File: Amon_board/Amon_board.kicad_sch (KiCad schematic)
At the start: 40 parts, among them J1 USB2.0_C_Rev, J2 Conn_2x5 pin, SW1 SW_DPDT, SW2 SW_SPST, U1 USBLC6-2P6, U2 STM32F405RGT6-LQFP64, U3 W25Q128JVS, Y1 25MHz

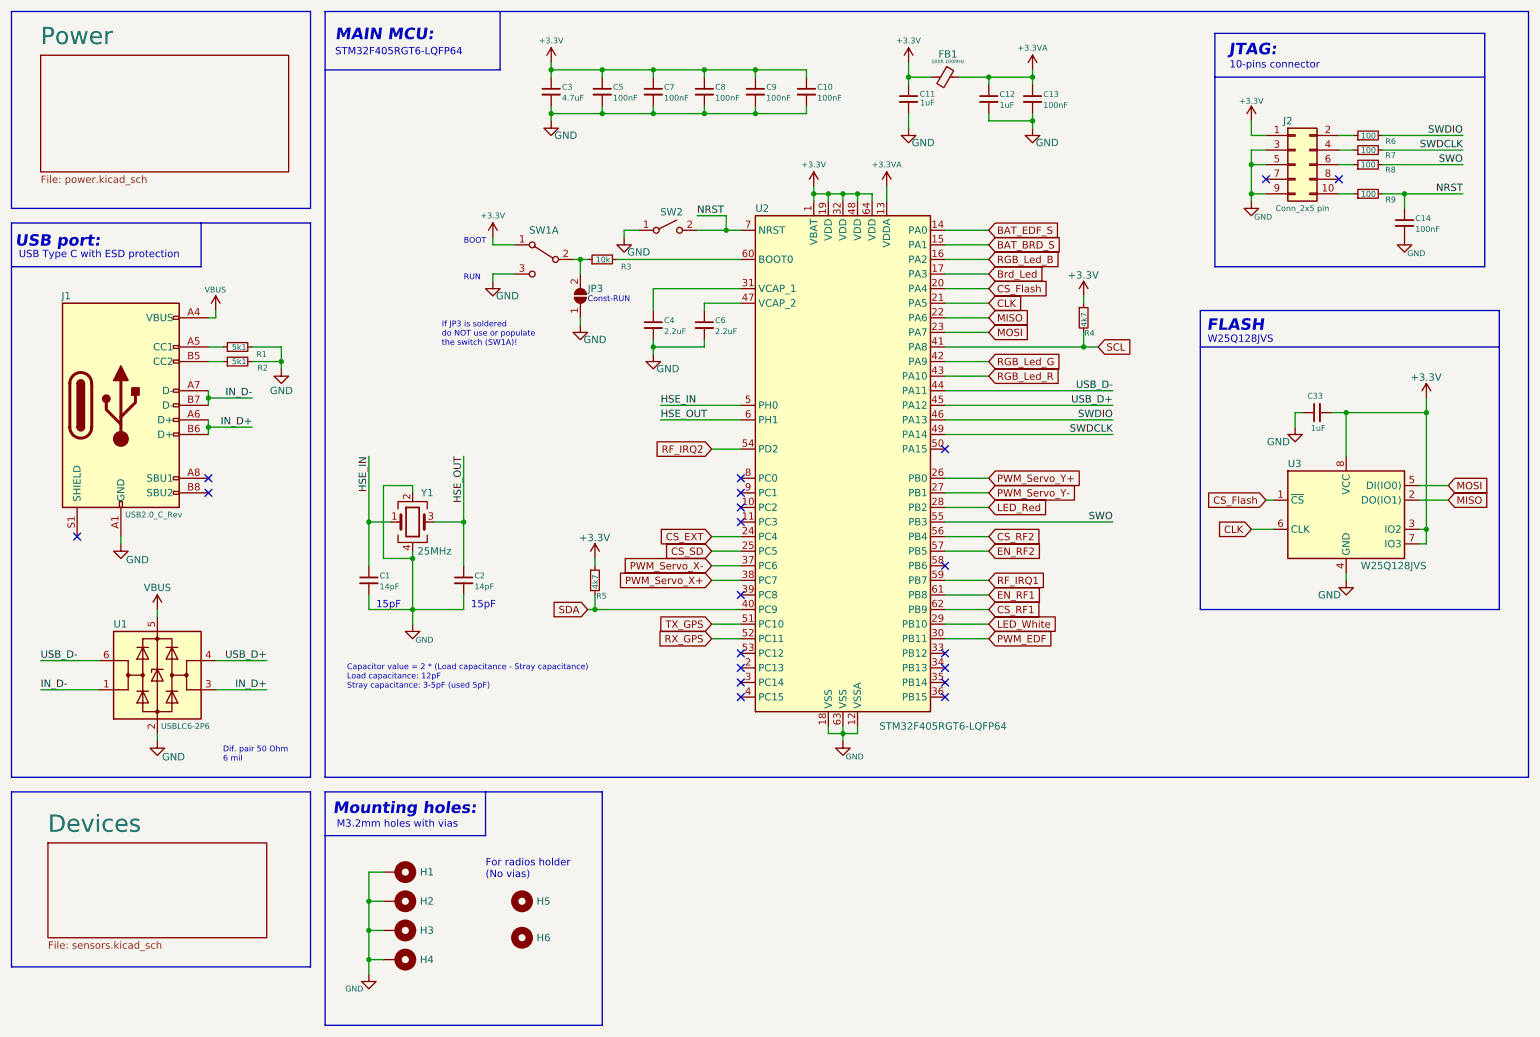
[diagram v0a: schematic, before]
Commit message: changed directories
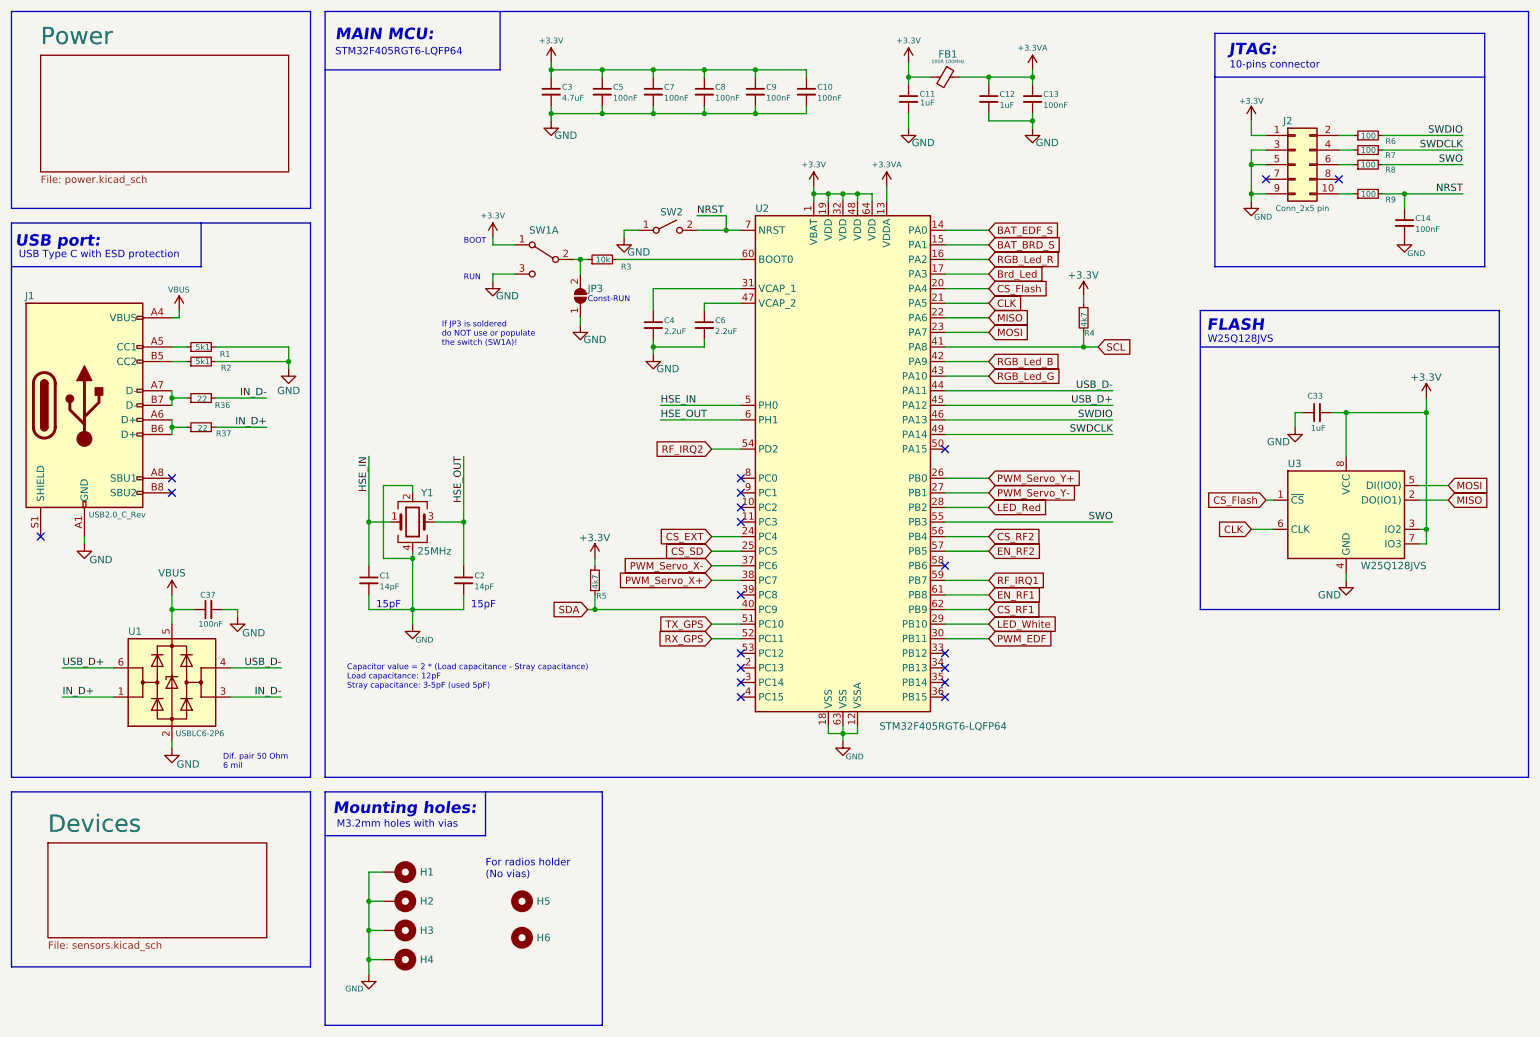
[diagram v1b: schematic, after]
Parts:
- added C37: 100nF, Capacitor_SMD:C_0603_1608Metric, symbol Device:C_Small
- added R36, R37: 22, Resistor_SMD:R_0603_1608Metric, symbol Device:R_Small
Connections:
- net GND: now also C37.2
- net IN_D+: now also U1.1 (I/O1), R37.2; no longer J1.A6 (D+), J1.B6 (D+), U1.3 (I/O2)
- net IN_D-: now also U1.3 (I/O2), R36.2; no longer J1.A7 (D-), J1.B7 (D-), U1.1 (I/O1)
- net RGB_Led_B: now also U2.42 (PA9); no longer U2.16 (PA2)
- net RGB_Led_G: now also U2.43 (PA10); no longer U2.42 (PA9)
- net RGB_Led_R: now also U2.16 (PA2); no longer U2.43 (PA10)
- net USB_D+: now also U1.6 (I/O1); no longer U1.4 (I/O2)
- net USB_D-: now also U1.4 (I/O2); no longer U1.6 (I/O1)
- net VBUS: now also C37.1
- new net: J1.A7 (D-), J1.B7 (D-), R36.1
- new net: J1.A6 (D+), J1.B6 (D+), R37.1
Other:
- moved on the sheet: J1, R1, R2, U1
